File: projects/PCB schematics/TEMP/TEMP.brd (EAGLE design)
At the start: 78.7 x 64.8 mm, 19 parts, among them IC1 4051D, IC10 4051D, IC2 4051D, IC3 4051D, IC4 4051D, IC5 4051D, IC6 4051D, IC7 4051D, IC8 4051D, IC9 4051D, J1 SAMTEC-TFM-120-02-X-D-LCJ, J2 SAMTEC-TFM-120-02-X-D-LCJ, X2 5566-4, X3 5566-2, X4 5566-10

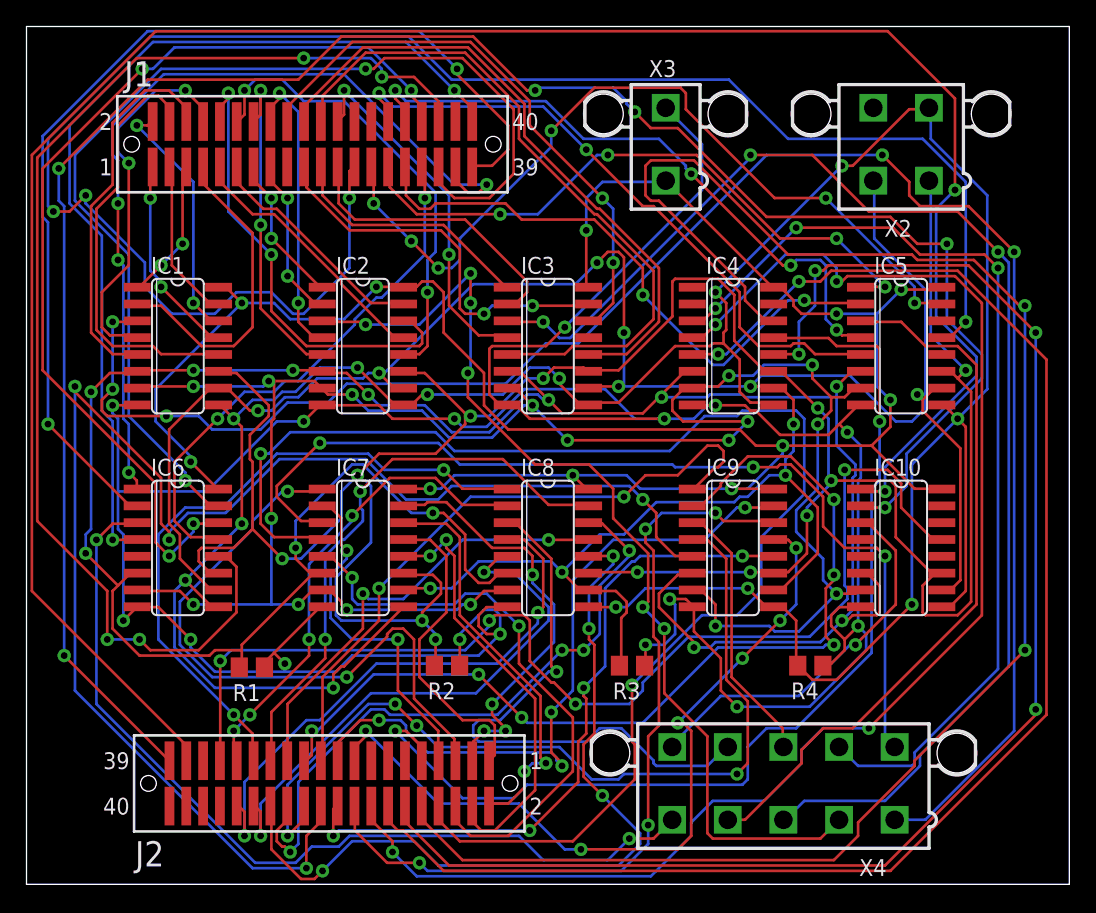
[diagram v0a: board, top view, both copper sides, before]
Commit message: TEMP - Initial board placement.
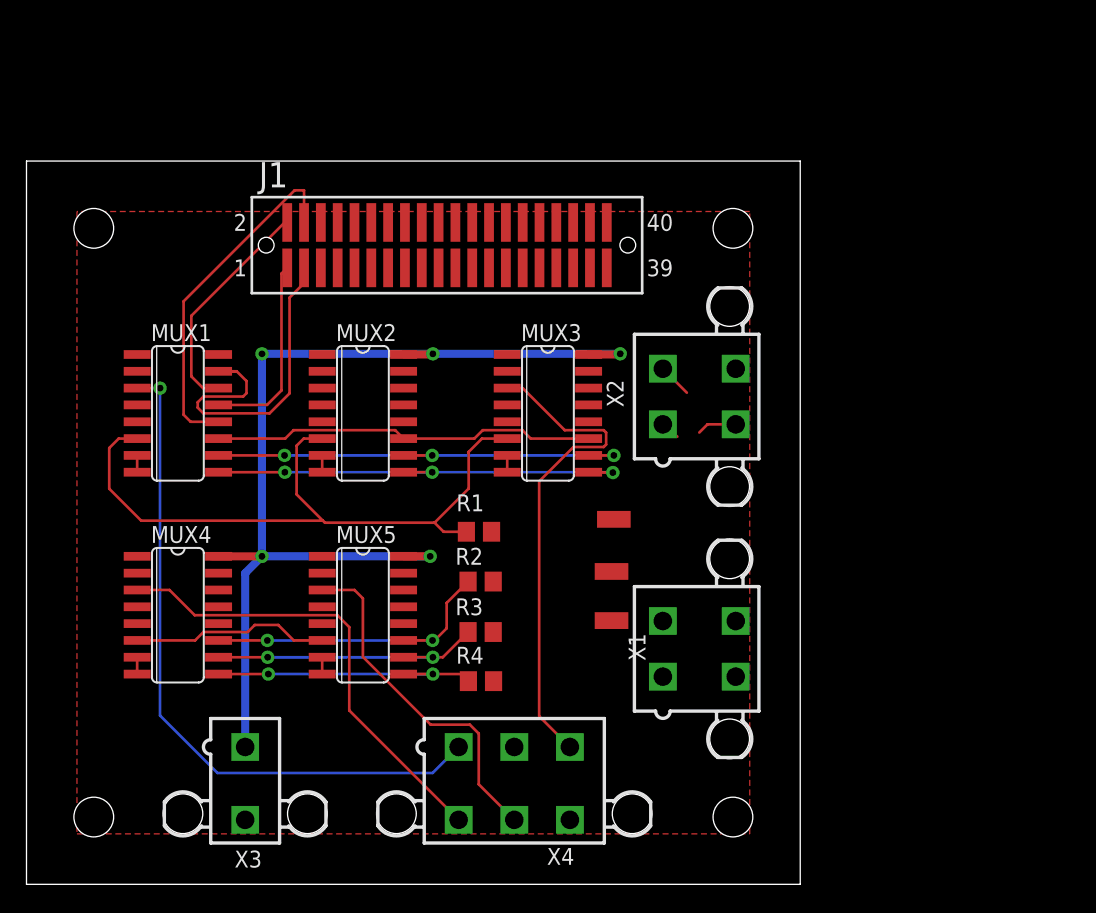
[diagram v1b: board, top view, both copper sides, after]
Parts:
- removed IC1, IC10, IC2, IC3, IC4, IC5, IC6, IC7, IC8, IC9: 4051D, 40xx:SO16
- removed J2: SAMTEC-TFM-120-02-X-D-LCJ, SAMTEC-TFM-120-02-X-D-LC:SAMTEC-TFM-120-02-X-D-LC
- added MUX1, MUX2, MUX3, MUX4, MUX5: 4051D, 40xx:SO16
- added SH1, SH2, SH3: SHORTT5, shorts:SHORT_TOP-50
- added X1: 5566-4, con-molex:5566-4
- R1, R2, R3, R4: value (none) -> 50k
- X4: value 5566-10 -> 5566-6; device con-molex:5566-10 -> con-molex:5566-6
- moved X3 57.8 mm to (16.5, 7.62), turned to 180 degrees
- moved R4 24.9 mm to (34.3, 15.3)
- moved X2 24.4 mm to (50.8, 36.8), turned to 270 degrees
- moved X4 20.3 mm to (36.8, 7.62), turned to 180 degrees
- moved R1 20.0 mm to (34.2, 26.6)
- moved J1 12.7 mm to (31.8, 48.3)
- moved R3 11.7 mm to (34.3, 19.1)
- moved R2 6.84 mm to (34.3, 22.9)
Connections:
- removed net CS_A: IC1.11, IC10.11, IC2.11, IC3.11, IC4.11, IC5.11, IC6.11, IC7.11, IC8.11, IC9.11, R2.2, X2.1
- removed net CS_B: IC1.10, IC10.10, IC2.10, IC3.10, IC4.10, IC5.10, IC6.10, IC7.10, IC8.10, IC9.10, R3.2, X2.2
- removed net CS_C: IC1.9, IC10.9, IC2.9, IC3.9, IC4.9, IC5.9, IC6.9, IC7.9, IC8.9, IC9.9, R4.2, X2.3
- removed net TEMP41: IC7.13, J2.1
- removed net TEMP42: IC7.14, J2.2
- removed net TEMP43: IC7.15, J2.3
- removed net TEMP44: IC7.12, J2.4
- removed net TEMP45: IC7.1, J2.5
- removed net TEMP46: IC7.5, J2.6
- removed net TEMP47: IC7.2, J2.7
- removed net TEMP48: IC7.4, J2.8
- removed net TEMP49: IC4.13, J2.9
- removed net TEMP50: IC4.14, J2.10
- removed net TEMP51: IC4.15, J2.11
- removed net TEMP52: IC4.12, J2.12
- removed net TEMP53: IC4.1, J2.13
- removed net TEMP54: IC4.5, J2.14
- removed net TEMP55: IC4.2, J2.15
- removed net TEMP56: IC4.4, J2.16
- removed net TEMP57: IC9.13, J2.17
- removed net TEMP58: IC9.14, J2.18
- removed net TEMP59: IC9.15, J2.19
- removed net TEMP60: IC9.12, J2.20
- removed net TEMP61: IC9.1, J2.21
- removed net TEMP62: IC9.5, J2.22
- removed net TEMP63: IC9.2, J2.23
- removed net TEMP64: IC9.4, J2.24
- removed net TEMP65: IC8.13, J2.25
- removed net TEMP66: IC8.14, J2.26
- removed net TEMP67: IC8.15, J2.27
- removed net TEMP68: IC8.12, J2.28
- removed net TEMP69: IC8.1, J2.29
- removed net TEMP70: IC8.5, J2.30
- removed net TEMP71: IC8.2, J2.31
- removed net TEMP72: IC8.4, J2.32
- removed net TEMP73: IC10.13, J2.33
- removed net TEMP74: IC10.14, J2.34
- removed net TEMP75: IC10.15, J2.35
- removed net TEMP76: IC10.12, J2.36
- removed net TEMP77: IC10.1, J2.37
- removed net TEMP78: IC10.5, J2.38
- removed net TEMP79: IC10.2, J2.39
- removed net TEMP80: IC10.4, J2.40
- removed net TEMP_OUT10: IC10.3, X4.10
- removed net TEMP_OUT6: IC7.3, X4.6
- removed net TEMP_OUT7: IC4.3, X4.7
- removed net TEMP_OUT8: IC9.3, X4.8
- removed net TEMP_OUT9: IC8.3, X4.9
- removed net VEE: IC1.7, IC10.7, IC2.7, IC3.7, IC4.7, IC5.7, IC6.7, IC7.7, IC8.7, IC9.7
- new net CS_A_IN: MUX1.11, MUX2.11, MUX3.11, MUX4.11, MUX5.11, R2.2, SH1.1, X2.1
- new net CS_A_OUT: SH1.2, X1.1
- new net CS_B_IN: MUX1.10, MUX2.10, MUX3.10, MUX4.10, MUX5.10, R3.2, SH2.1, X2.2
- new net CS_B_OUT: SH2.2, X1.2
- new net CS_C_IN: MUX1.9, MUX2.9, MUX3.9, MUX4.9, MUX5.9, R4.2, SH3.1, X2.3
- new net CS_C_OUT: SH3.2, X1.3
- net GND: now also MUX1.7, MUX1.8, MUX2.7, MUX2.8, MUX3.7, MUX3.8, MUX4.7, MUX4.8, MUX5.7, MUX5.8; no longer IC1.8, IC10.8, IC2.8, IC3.8, IC4.8, IC5.8, IC6.8, IC7.8, IC8.8, IC9.8
- net INH: now also MUX1.6, MUX2.6, MUX3.6, MUX4.6, MUX5.6; no longer IC1.6, IC10.6, IC2.6, IC3.6, IC4.6, IC5.6, IC6.6, IC7.6, IC8.6, IC9.6
- net TEMP1: now also MUX1.13; no longer IC1.13
- net TEMP10: now also MUX2.14; no longer IC2.14
- net TEMP11: now also MUX2.15; no longer IC2.15
- net TEMP12: now also MUX2.12; no longer IC2.12
- net TEMP13: now also MUX2.1; no longer IC2.1
- net TEMP14: now also MUX2.5; no longer IC2.5
- net TEMP15: now also MUX2.2; no longer IC2.2
- net TEMP16: now also MUX2.4; no longer IC2.4
- net TEMP17: now also MUX3.13; no longer IC3.13
- net TEMP18: now also MUX3.14; no longer IC3.14
- net TEMP19: now also MUX3.15; no longer IC3.15
- net TEMP2: now also MUX1.14; no longer IC1.14
- net TEMP20: now also MUX3.12; no longer IC3.12
- net TEMP21: now also MUX3.1; no longer IC3.1
- net TEMP22: now also MUX3.5; no longer IC3.5
- net TEMP23: now also MUX3.2; no longer IC3.2
- net TEMP24: now also MUX3.4; no longer IC3.4
- net TEMP25: now also MUX4.13; no longer IC5.13
- net TEMP26: now also MUX4.14; no longer IC5.14
- net TEMP27: now also MUX4.15; no longer IC5.15
- net TEMP28: now also MUX4.12; no longer IC5.12
- net TEMP29: now also MUX4.1; no longer IC5.1
- net TEMP3: now also MUX1.15; no longer IC1.15
- net TEMP30: now also MUX4.5; no longer IC5.5
- net TEMP31: now also MUX4.2; no longer IC5.2
- net TEMP32: now also MUX4.4; no longer IC5.4
- net TEMP33: now also MUX5.13; no longer IC6.13
- net TEMP34: now also MUX5.14; no longer IC6.14
- net TEMP35: now also MUX5.15; no longer IC6.15
- net TEMP36: now also MUX5.12; no longer IC6.12
- net TEMP37: now also MUX5.1; no longer IC6.1
- net TEMP38: now also MUX5.5; no longer IC6.5
- net TEMP39: now also MUX5.2; no longer IC6.2
- net TEMP4: now also MUX1.12; no longer IC1.12
- net TEMP40: now also MUX5.4; no longer IC6.4
- net TEMP5: now also MUX1.1; no longer IC1.1
- net TEMP6: now also MUX1.5; no longer IC1.5
- net TEMP7: now also MUX1.2; no longer IC1.2
- net TEMP8: now also MUX1.4; no longer IC1.4
- net TEMP9: now also MUX2.13; no longer IC2.13
- net TEMP_OUT1: now also MUX1.3; no longer IC1.3
- net TEMP_OUT2: now also MUX2.3; no longer IC2.3
- net TEMP_OUT3: now also MUX3.3; no longer IC3.3
- net TEMP_OUT4: now also MUX4.3; no longer IC5.3
- net TEMP_OUT5: now also MUX5.3; no longer IC6.3
- net VCC: now also MUX1.16, MUX2.16, MUX3.16, MUX4.16, MUX5.16; no longer IC1.16, IC10.16, IC2.16, IC3.16, IC4.16, IC5.16, IC6.16, IC7.16, IC8.16, IC9.16
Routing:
- net GND: track 240.1 -> 6.35 mm, vias 16 -> 0
- net CS_C: track 215.0 -> 0.00 mm, vias 13 -> 0
- net CS_A: track 205.5 -> 0.00 mm, vias 12 -> 0
- net CS_B: track 199.0 -> 0.00 mm, vias 11 -> 0
- net TEMP77: track 162.7 -> 0.00 mm, vias 2 -> 0
- net VEE: track 158.2 -> 0.00 mm, vias 17 -> 0
- net TEMP79: track 152.1 -> 0.00 mm, vias 6 -> 0
- net TEMP25: track 134.1 -> 0.00 mm, vias 4 -> 0
- net TEMP50: track 131.0 -> 0.00 mm, vias 2 -> 0
- net INH: track 187.8 -> 67.2 mm, vias 12 -> 0
- net TEMP54: track 116.3 -> 0.00 mm, vias 2 -> 0
- net TEMP62: track 113.0 -> 0.00 mm, vias 4 -> 0
- net TEMP52: track 111.4 -> 0.00 mm, vias 4 -> 0
- net TEMP56: track 109.3 -> 0.00 mm, vias 4 -> 0
- net TEMP48: track 107.0 -> 0.00 mm, vias 2 -> 0
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- added copper zone on layer 1, net GND
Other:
- board size 78.7 x 64.8 mm -> 58.4 x 54.6 mm
